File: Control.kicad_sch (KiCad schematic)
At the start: 8 parts, among them U1 XC95144XL-TQ100

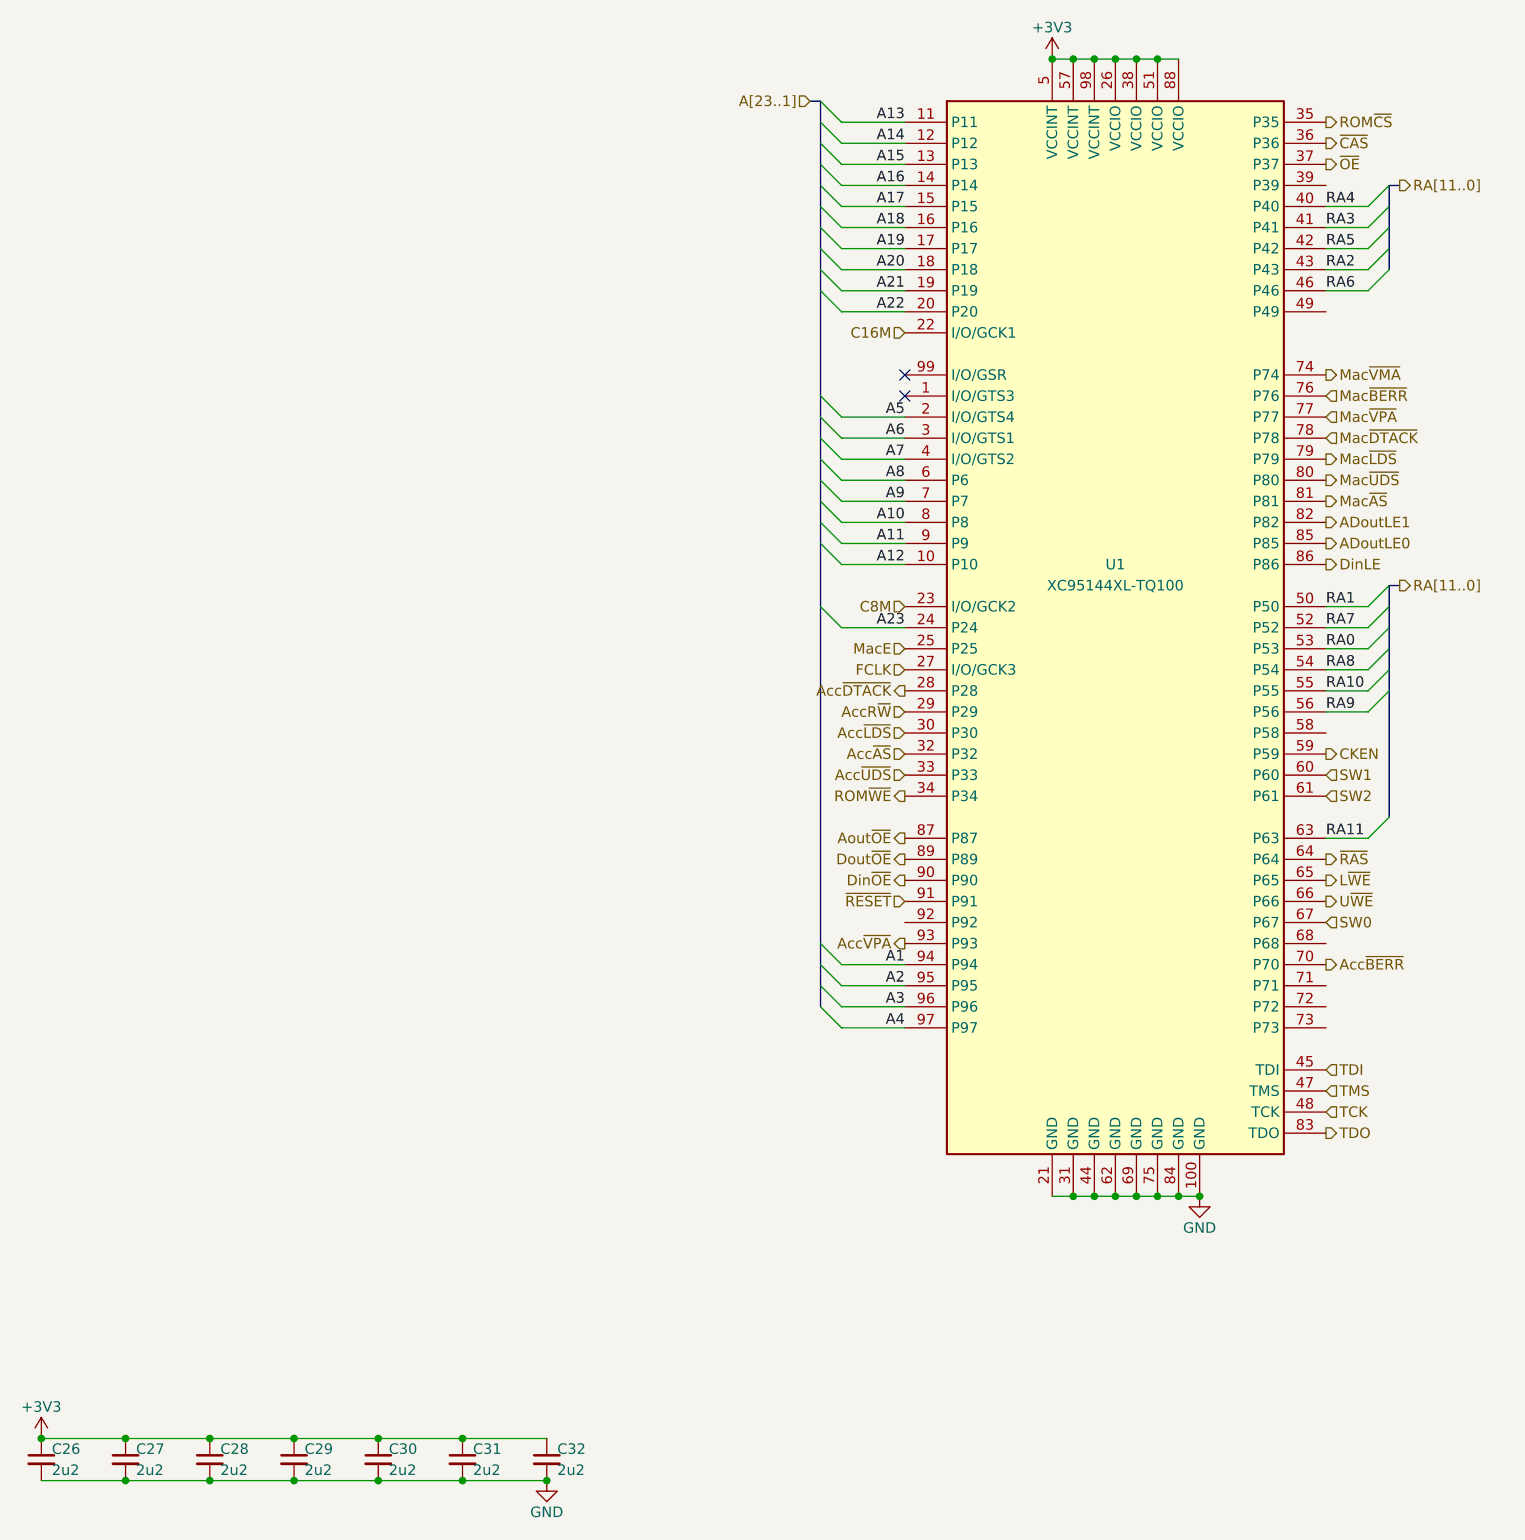
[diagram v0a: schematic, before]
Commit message: Prototype
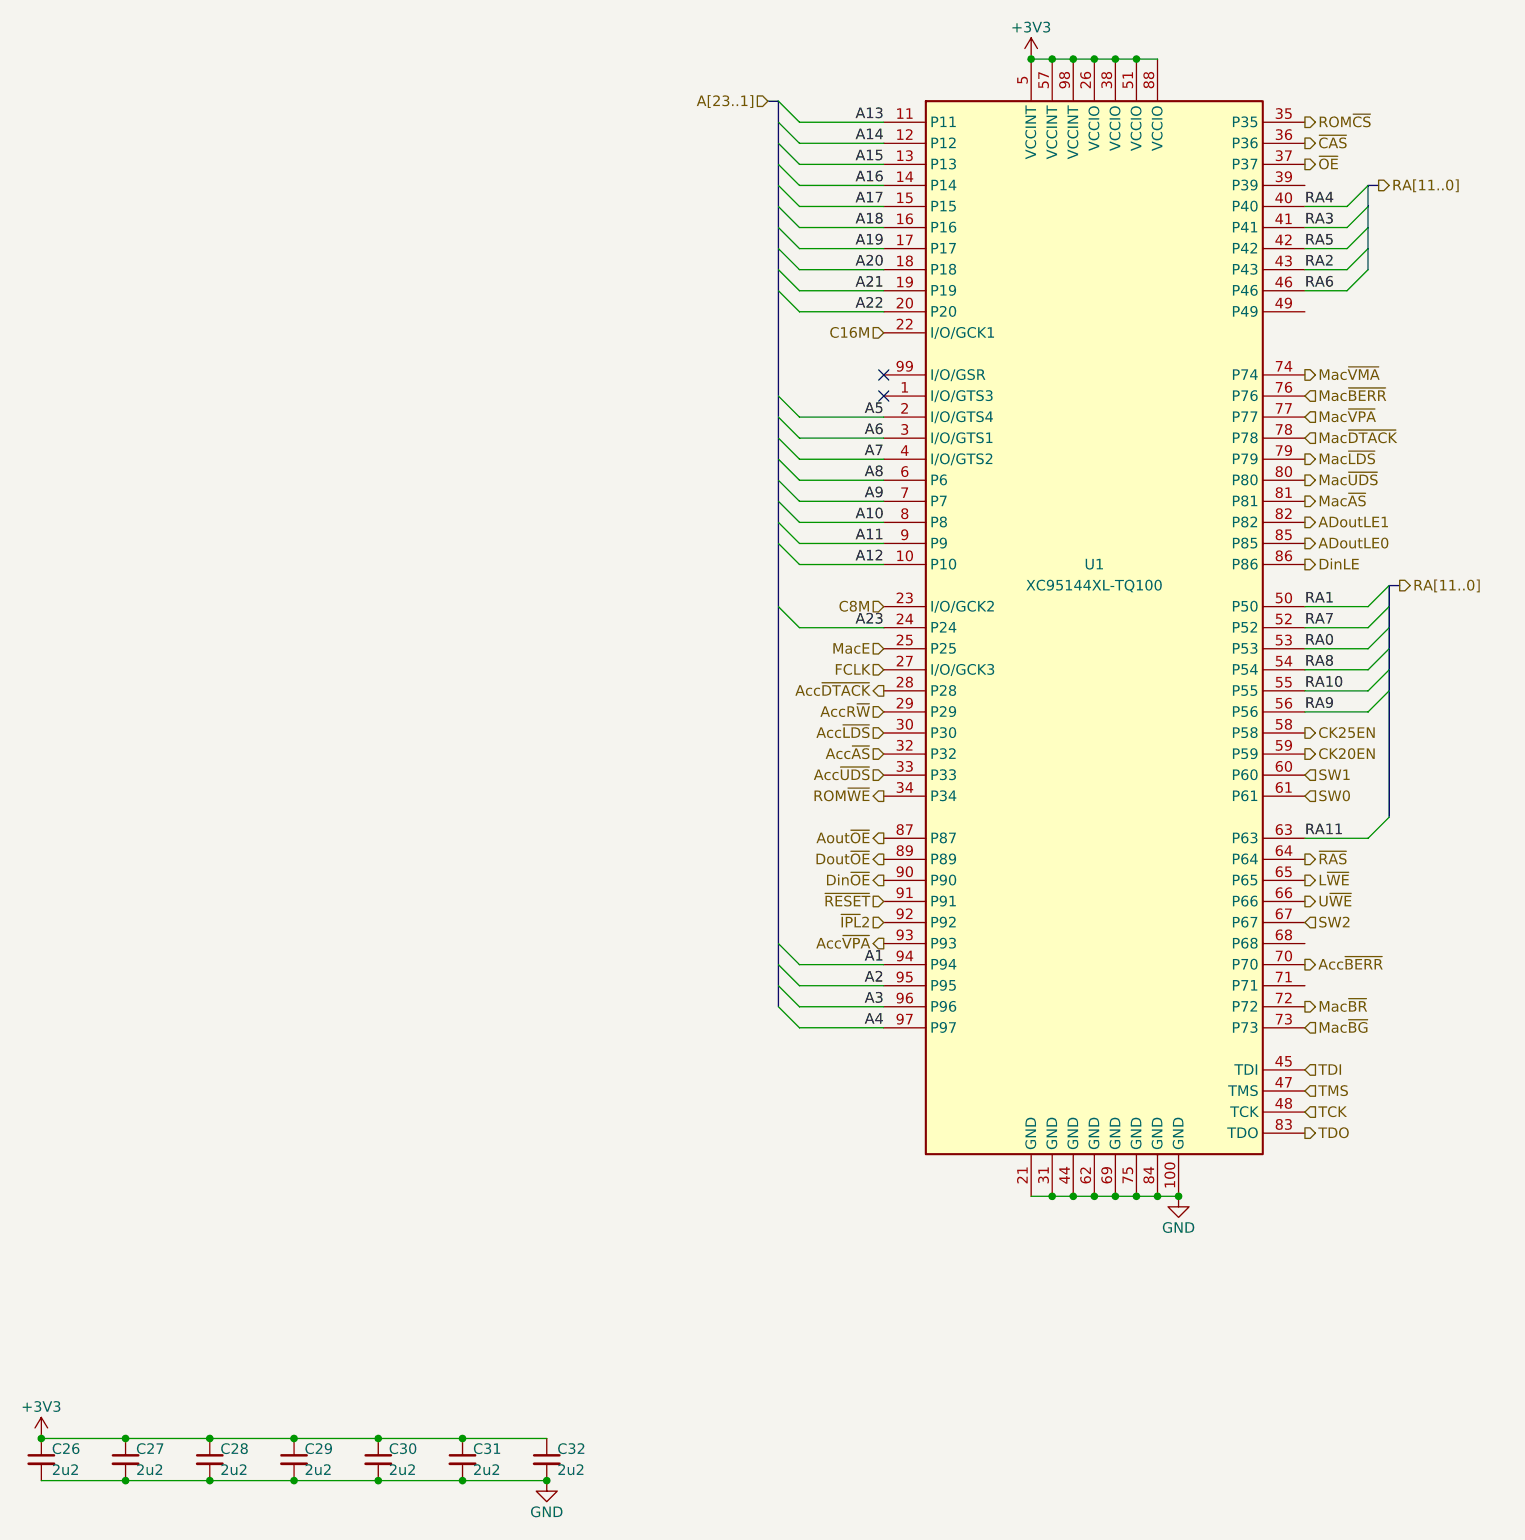
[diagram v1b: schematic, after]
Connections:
- net SW0: now also U1.61 (P61); no longer U1.67 (P67)
- net SW2: now also U1.67 (P67); no longer U1.61 (P61)
- net CK25EN: now reaches U1.58 (P58)
- net Mac~{BR}: now reaches U1.72 (P72)
- net Mac~{BG}: now reaches U1.73 (P73)
- net ~{IPL}2: now reaches U1.92 (P92)
- net CKEN renamed CK20EN
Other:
- moved on the sheet: U1

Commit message: Toward final "A"
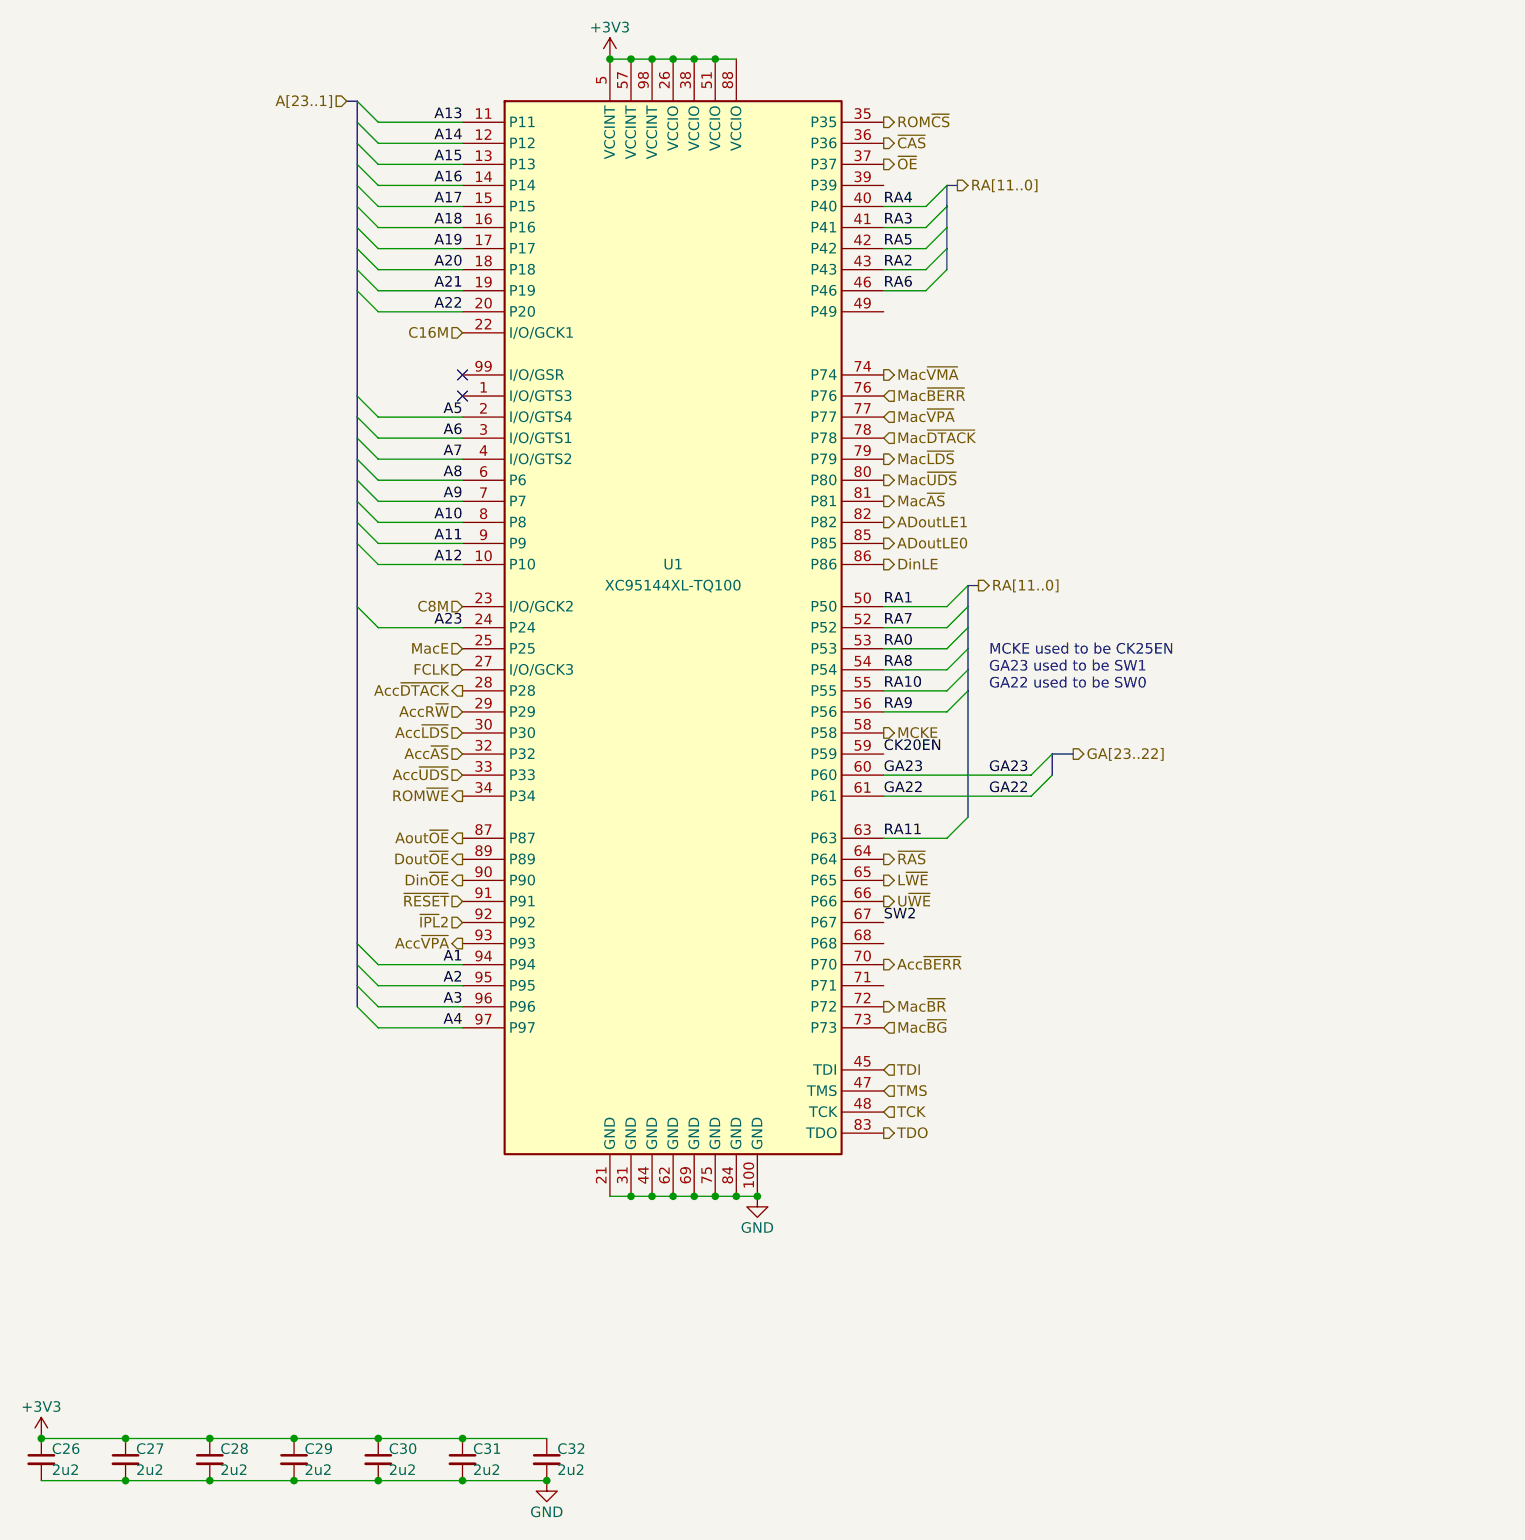
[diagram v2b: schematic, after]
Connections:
- net CK25EN renamed MCKE
- net SW0 renamed GA22
- net SW1 renamed GA23
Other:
- note added: "MCKE used to be CK25EN GA23 used to be SW1 GA22 used to be SW0"
- moved on the sheet: U1
